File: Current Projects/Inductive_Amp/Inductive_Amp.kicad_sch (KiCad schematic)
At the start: 26 parts, among them J1 INPUT, J2 OUTPUT, U1 NA555D, U2 74LS14, U3 TLV2372

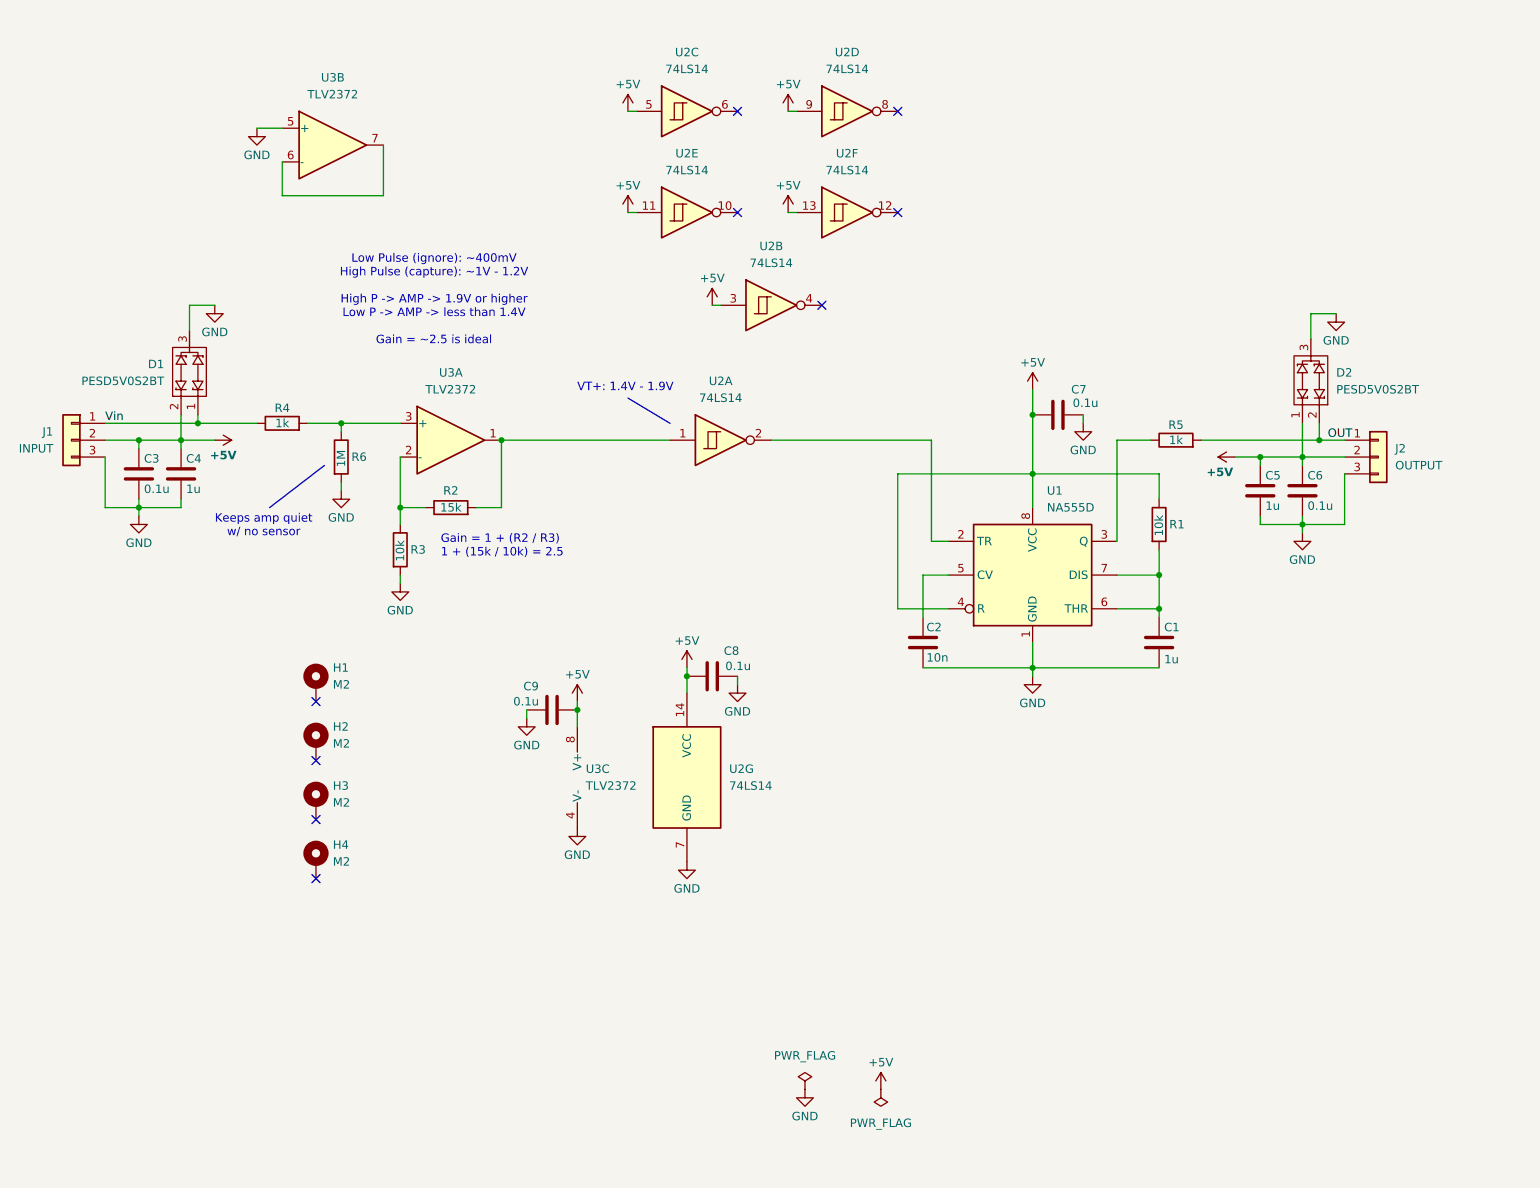
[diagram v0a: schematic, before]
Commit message: Inductive amp fab files
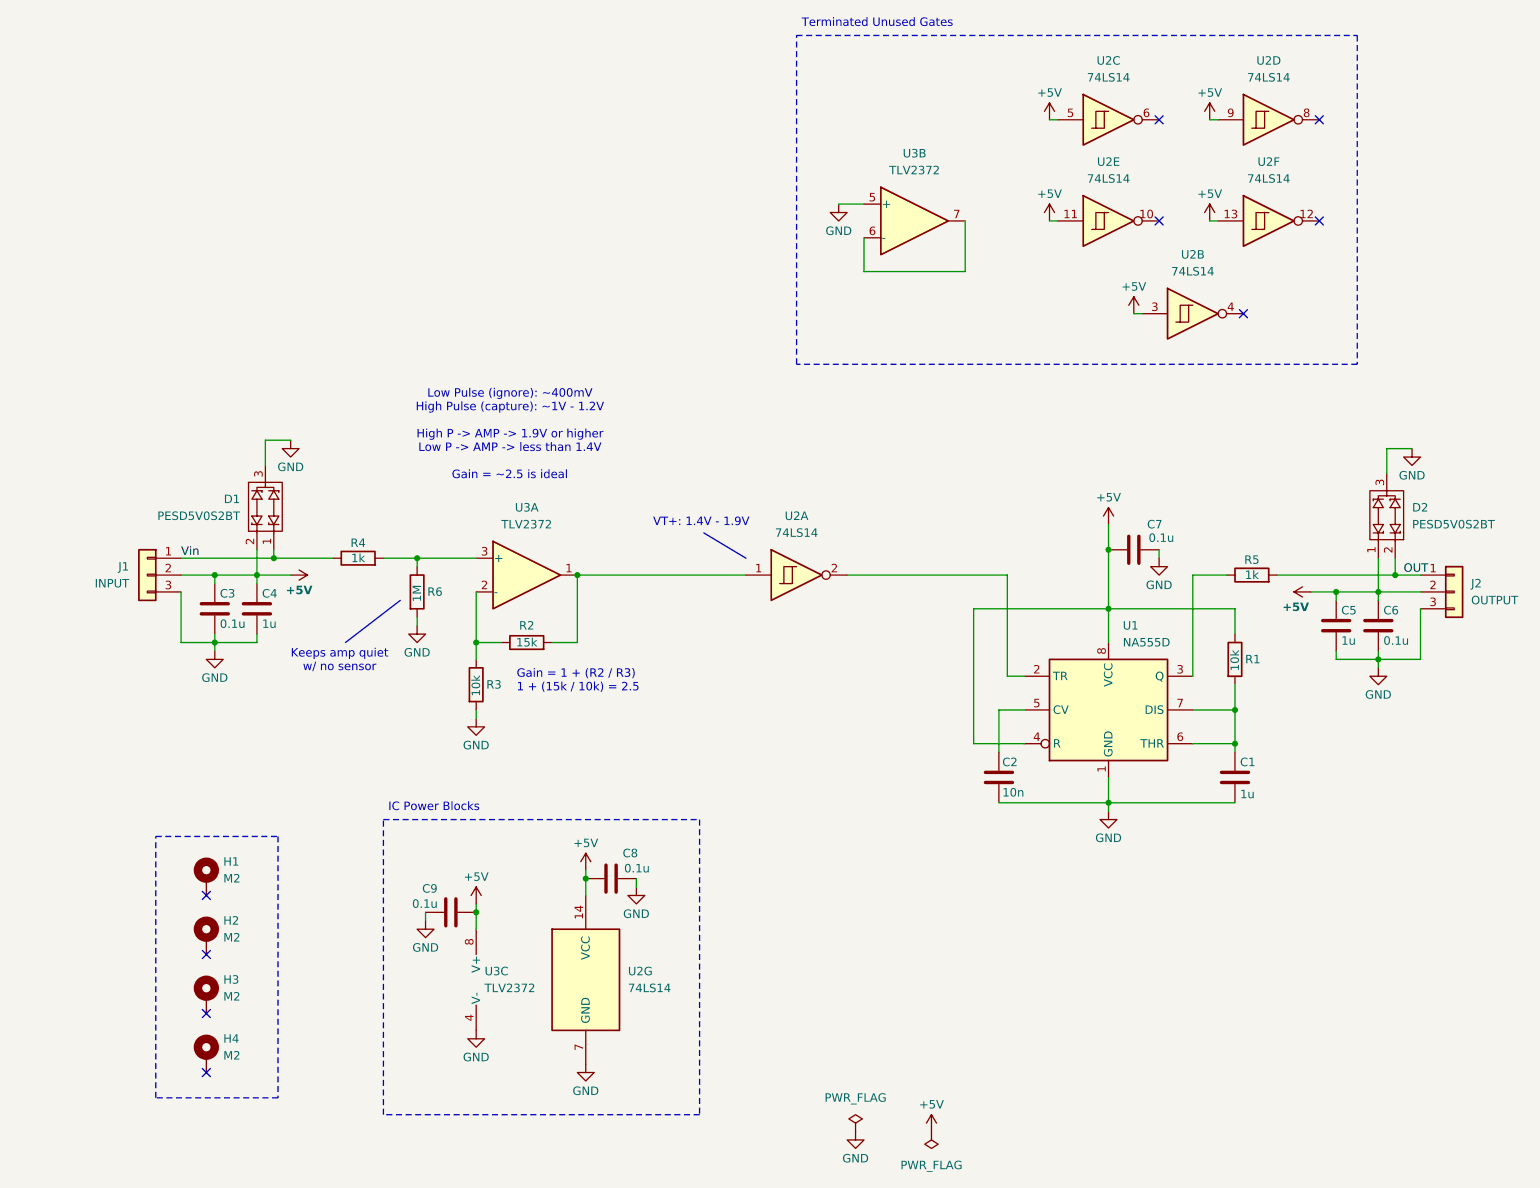
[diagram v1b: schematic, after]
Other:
- note added: "IC Power Blocks"
- note added: "Terminated Unused Gates"
- moved on the sheet: C1, C2, C3, C4, C5, C6, C7, C8, C9, D1, D2, H1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
